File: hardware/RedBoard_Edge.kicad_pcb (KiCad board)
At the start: 2 copper layers, 101.6 x 38.1 mm, 56 parts, among them J1 CONN_025MM, J17 QWIIC_CONNECTORJS-1MM, J2 CONN_03X2SMT, J4 USB_MICRO-B_FEMALE-SMT, J5 CONN_04, J6 CONN_04, Q1 MOSFET_PCH-SI2309DS, Q2 MOSFET-NCH-BSS138, U1 CH340GSMD, U2 V_REG_MIC52053.3V, U3 Standoff_Grounding, U4 ATMEGA328P_TQFP, U5 Standoff_Grounding, U6 V_REG_LM1117SOT223, Y1 RESONATOR-16MHZSMD_3.2X1.3, Y2 CRYSTAL-12MHZ

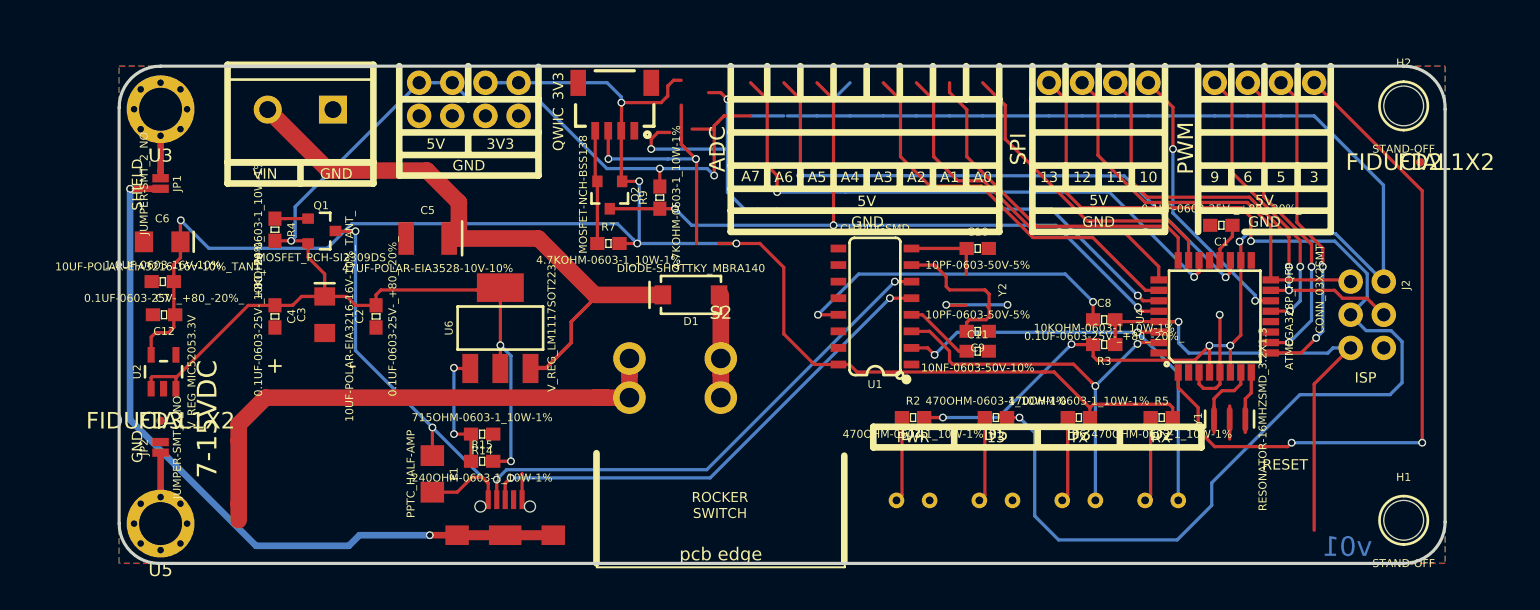
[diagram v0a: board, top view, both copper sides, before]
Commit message: v02
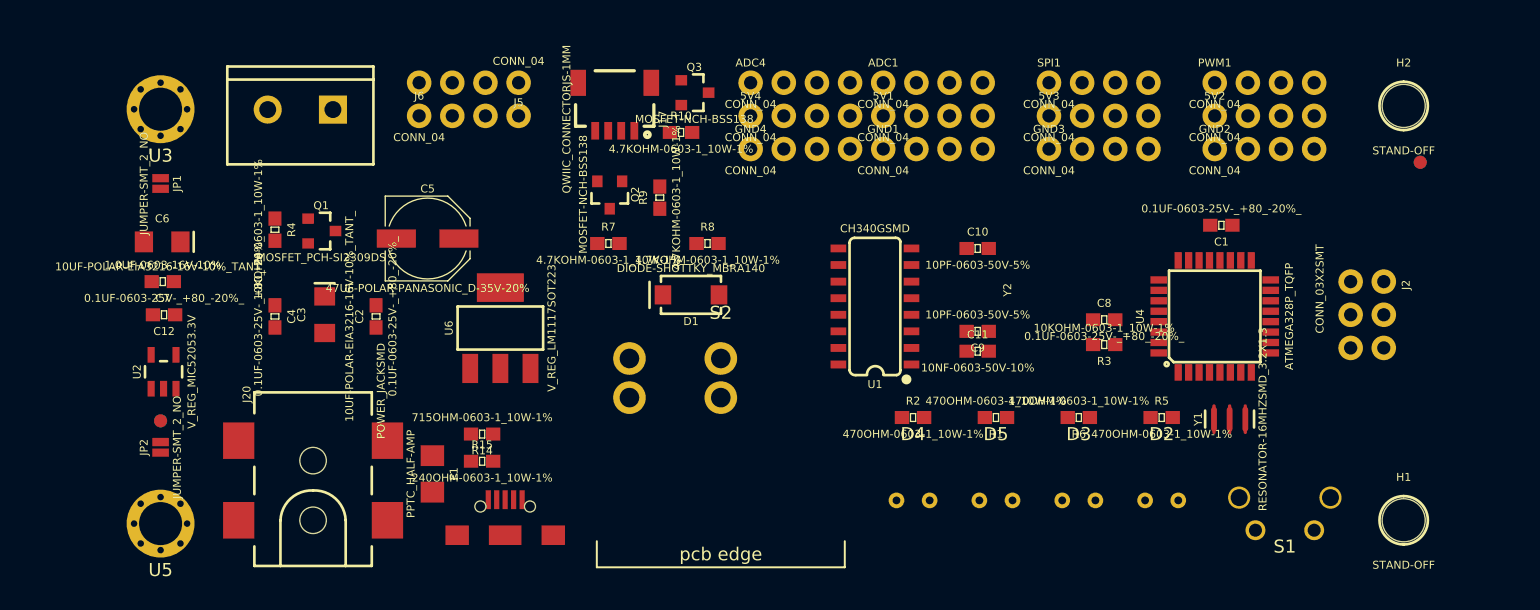
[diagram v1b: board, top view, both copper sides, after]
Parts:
- added 5V1: CONN_04, Connectors:1X04_NO_SILK, F.Cu at (159.5, 83.1)
- added 5V2: CONN_04, Connectors:1X04_NO_SILK, F.Cu at (184.9, 83.1)
- added 5V3: CONN_04, Connectors:1X04_NO_SILK, F.Cu at (172.2, 83.1)
- added 5V4: CONN_04, Connectors:1X04_NO_SILK, F.Cu at (149.4, 83.1)
- added ADC1: CONN_04, Connectors:1X04_NO_SILK, F.Cu at (159.5, 80.5)
- added ADC4: CONN_04, Connectors:1X04_NO_SILK, F.Cu at (149.4, 80.5)
- added GND1: CONN_04, Connectors:1X04_NO_SILK, F.Cu at (159.5, 85.6)
- added GND2: CONN_04, Connectors:1X04_NO_SILK, F.Cu at (184.9, 85.6)
- added GND3: CONN_04, Connectors:1X04_NO_SILK, F.Cu at (172.2, 85.6)
- added GND4: CONN_04, Connectors:1X04_NO_SILK, F.Cu at (149.4, 85.6)
- added J20: POWER_JACKSMD, Connectors:POWER_JACK_SMD_GND, F.Cu at (115.8, 114.0)
- added LOGO1: SFE_LOGO_NAME_FLAME.1_INCH, Aesthetics:SFE_LOGO_NAME_FLAME_.1, B.Cu at (123.4, 95.2)
- added Q3: MOSFET-NCH-BSS138, Silicon-Standard:SOT23-3, F.Cu at (145.0, 81.3)
- added R10: 4.7KOHM-0603-1_10W-1%, Resistors:0603, F.Cu at (144.0, 84.3)
- added R8: 4.7KOHM-0603-1_10W-1%, Resistors:0603, F.Cu at (146.1, 92.8)
- added S1: MOMENTARY-SWITCH-SPST-2-PTH-RT-ANGLE, Switches:SWITCH TACTILE SPST-NO 0.05A 12V, F.Cu at (190.3, 112.3)
- C5: value 47UF-POLAR-EIA3528-10V-10% -> 47UF-POLAR-PANASONIC_D-35V-20%; footprint Capacitors:EIA3528 -> Capacitors:PANASONIC_D
- FD1, FD2, FD3, FD4: footprint Aesthetics:FIDUCIAL-MICRO -> Aesthetics:FIDUCIAL-1X2
- H1, H2: footprint Hardware:STAND-OFF-TIGHT -> Hardware:STAND-OFF
- J17: footprint SparkX:SparkX-1X04_1MM_RA -> Connectors:1X04_1MM_RA
- J5, J6, PWM1, SPI1: footprint Connectors:1X04 -> Connectors:1X04_NO_SILK
- LOGO2: footprint OSHW-LOGO-S -> Aesthetics:OSHW-LOGO-S
- Y2: footprint Clocks:CRYSTAL-SMD-3.2X2.5MM -> Clocks:CRYSTAL-SMD-5X3.2-4PAD
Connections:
- Q1 pad 1: Net-(J20-PadP$4) -> GND
- R4 pad 1: Net-(J20-PadP$4) -> GND
- U4 pad 17: Net-(U4-Pad17) -> /SCK
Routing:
- net 5V: track 218.1 -> 0.00 mm, vias 10 -> 0
- net 3.3V: track 132.3 -> 0.00 mm, vias 5 -> 0
- net /SCK: track 91.2 -> 0.00 mm, vias 2 -> 0
- net VIN: track 67.3 -> 0.00 mm
- net /HI_SDA: track 63.4 -> 0.00 mm, vias 3 -> 0
- net /usb_shield: track 60.5 -> 0.00 mm, vias 2 -> 0
- net /HI_SCL: track 56.8 -> 0.00 mm, vias 3 -> 0
- net /PWM3: track 53.9 -> 0.00 mm, vias 2 -> 0
- net /AD7: track 45.3 -> 0.00 mm, vias 2 -> 0
- net /AD6: track 44.9 -> 0.00 mm, vias 2 -> 0
- net Net-(J20-PadVIN0): track 42.0 -> 0.00 mm
- net Net-(J4-PadD-): track 39.6 -> 0.00 mm, vias 2 -> 0
- net Net-(J4-PadD+): track 38.3 -> 0.00 mm, vias 2 -> 0
- net /RESET: track 37.2 -> 0.00 mm, vias 1 -> 0
- net /MOSI: track 35.4 -> 0.00 mm, vias 2 -> 0
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- removed copper zone on B.Cu, net GND
- removed copper zone on F.Cu, net GND
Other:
- board outline removed
- board text removed: "+"
- board text removed: "-"
- board text removed: "10"
- board text removed: "11"
- board text removed: "12"
- board text removed: "13"
- board text removed: "3"
- board text removed: "3V3"
- board text removed: "5"
- board text removed: "5V"
- board text removed: "6"
- board text removed: "7-15VDC"
- board text removed: "9"
- board text removed: "A0"
- board text removed: "A1"
- board text removed: "A2"
- board text removed: "A3"
- board text removed: "A4"
- board text removed: "A5"
- board text removed: "A6"
- board text removed: "A7"
- board text removed: "ADC"
- board text removed: "Designed by: Nick Poole"
- board text removed: "GND"
- board text removed: "ISP"
- board text removed: "PWM"
- board text removed: "PWR"
- board text removed: "QWIIC"
- board text removed: "RESET"
- board text removed: "ROCKER SWITCH"
- board text removed: "RX"
- board text removed: "RedBoard Edge"
- board text removed: "Revised by: Andy England"
- board text removed: "SHIELD"
- board text removed: "SPI"
- board text removed: "Standoff O.C."
- board text removed: "TX"
- board text removed: "VIN"
- board text removed: "v01"
